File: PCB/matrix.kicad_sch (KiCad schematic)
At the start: 99 parts, among them SW10 EC_SW, SW100 EC_SW, SW11 EC_SW, SW12 EC_SW, SW13 EC_SW, SW14 EC_SW, SW15 EC_SW, SW16 EC_SW, SW17 EC_SW, SW18 EC_SW, SW19 EC_SW, SW2 EC_SW, SW20 EC_SW, SW21 EC_SW, SW22 EC_SW, SW23 EC_SW, SW24 EC_SW, SW25 EC_SW, SW26 EC_SW, SW27 EC_SW, SW28 EC_SW, SW29 EC_SW, SW3 EC_SW, SW30 EC_SW, SW31 1U, SW32 2U, SW33 1U, SW34 EC_SW, SW35 EC_SW, SW36 EC_SW, SW37 EC_SW, SW38 EC_SW, SW39 EC_SW, SW4 EC_SW, SW40 EC_SW, SW41 EC_SW, SW42 EC_SW, SW43 EC_SW, SW44 EC_SW, SW45 EC_SW, SW46 EC_SW, SW47 EC_SW, SW48 EC_SW, SW49 EC_SW, SW5 EC_SW, SW50 ANSI_\, SW51 ANSI_Enter, SW52 EC_SW, SW53 EC_SW, SW54 EC_SW, SW55 EC_SW, SW56 EC_SW, SW57 EC_SW, SW58 EC_SW, SW59 EC_SW, SW6 EC_SW, SW60 EC_SW, SW61 EC_SW, SW62 EC_SW, SW63 EC_SW, SW64 EC_SW, SW65 EC_SW, SW66 EC_SW, SW67 ISO_|, SW68 ANSI_Enter, SW69 1.25U, SW7 EC_SW, SW70 2.25U, SW71 1U, SW72 EC_SW, SW73 EC_SW, SW74 EC_SW, SW75 EC_SW, SW76 EC_SW, SW77 EC_SW, SW78 EC_SW, SW79 EC_SW, SW8 EC_SW, SW80 EC_SW, SW81 EC_SW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

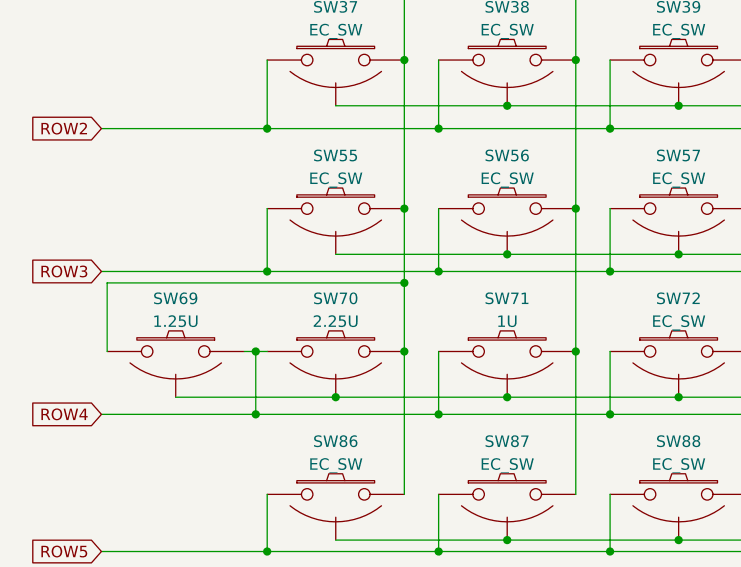
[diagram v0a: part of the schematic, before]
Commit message: Update
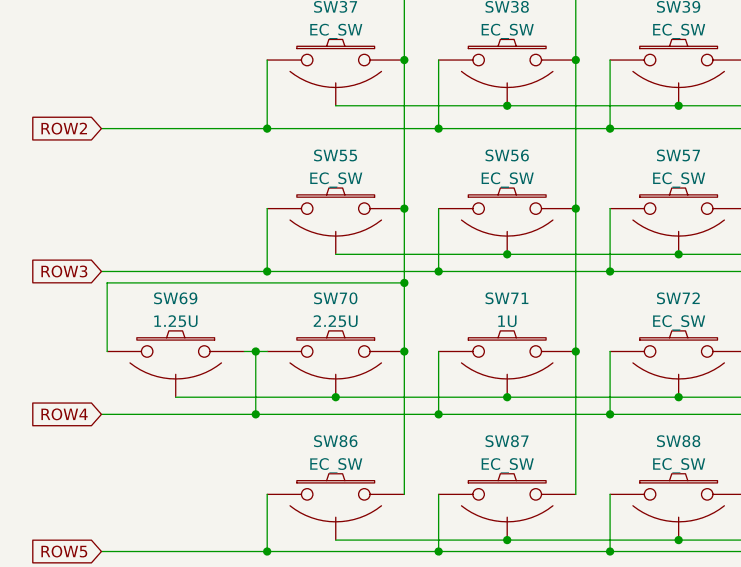
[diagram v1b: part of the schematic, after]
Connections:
- net COL0: now also SW55.1, SW70.1; no longer SW55.2, SW70.2
- net ROW3: now also SW55.2; no longer SW55.1
- net ROW4: now also SW70.2; no longer SW70.1
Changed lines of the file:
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@@
     (pin "3")
   )
-  (symbol (lib_id "cipulot_parts:EC_SW") (at 46.355 165.1 0) (unit 1)
+  (symbol (lib_id "cipulot_parts:EC_SW") (at 46.355 165.1 0) (mirror y) (unit 1)
     (in_bom yes) (on_board yes) (fields_autoplaced)
     (property "Reference" "SW70" (id 0) (at 46.355 159.2412 0))
@@
     (pin "1")
   )
-  (symbol (lib_id "cipulot_parts:EC_SW") (at 46.355 149.225 0) (unit 1)
+  (symbol (lib_id "cipulot_parts:EC_SW") (at 46.355 149.225 0) (mirror y) (unit 1)
     (in_bom yes) (on_board yes) (fields_autoplaced)
     (property "Reference" "SW55" (id 0) (at 46.355 143.3662 0))
